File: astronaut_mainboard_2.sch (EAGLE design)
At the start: 32 parts, among them IC1 ADUM1250, IC2 741G3157DBVR, IC3 741G3157DBVR, J1 User Interface (I2C), J2 Arduino Mega (UART), J3 HF Comm (UART), J4 User Interface (I2C), J5 GNSS (UART), Q1 BSS138, Q2 BSS138, Q3 BSS138, Q4 BSS138

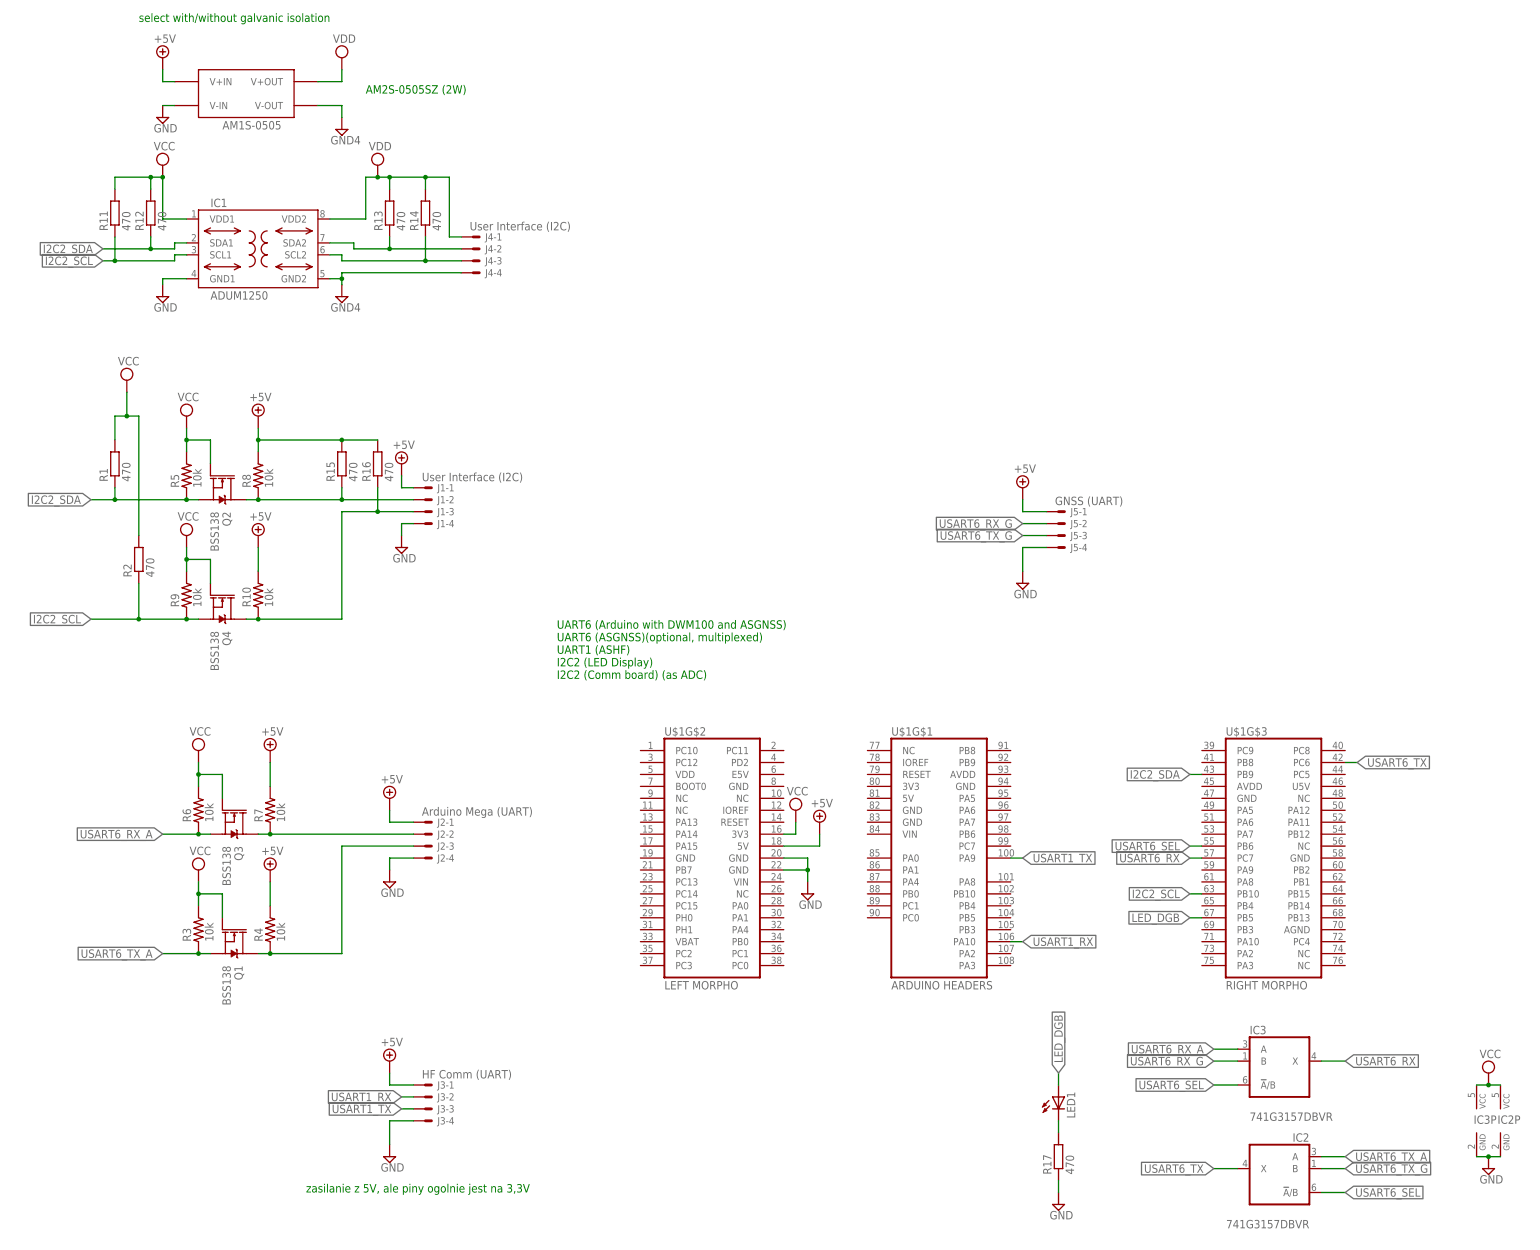
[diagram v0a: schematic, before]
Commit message: minor updates
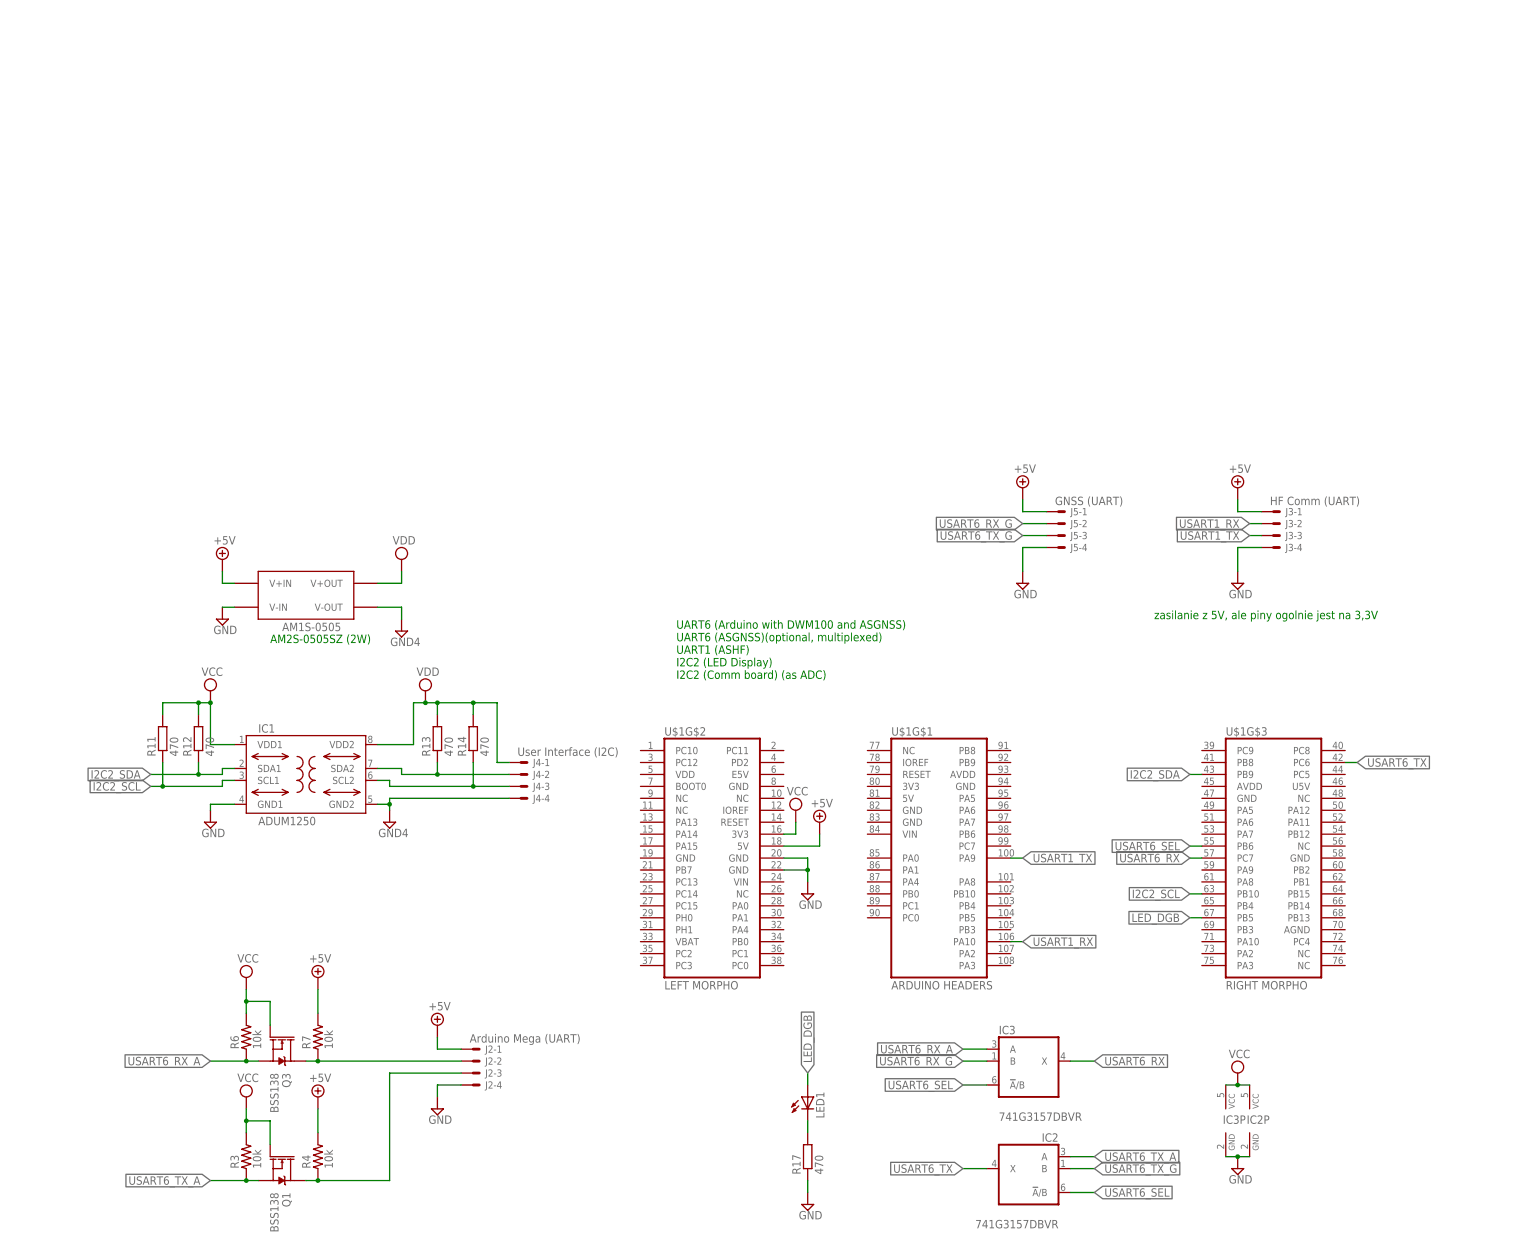
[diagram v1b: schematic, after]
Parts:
- removed J1: User Interface (I2C), EP_molex_6410_7395:22-05-7048-04
- removed Q2, Q4: BSS138, SparkFun-DiscreteSemi:MOSFET-NCH-AO3404A
- removed R1, R15, R16, R2: 470, rcl:R-EU_R0805
- removed R10, R5, R8, R9: 10k, rc-master-smd:R_1206
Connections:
- removed net ARDU_PIN_3: J1-2.S, Q2.D, R15.1, R8.1
- removed net ARDU_PIN_4: J1-3.S, Q4.D, R10.1, R16.1
- net +5V: no longer J1-1.S, R10.2, R15.2, R16.2, R8.2
- net GND: no longer J1-4.S
- net I2C2_SCL: no longer Q4.S, R2.1, R9.1
- net I2C2_SDA: no longer Q2.S, R1.1, R5.1
- net VCC: no longer Q2.G, Q4.G, R1.2, R2.2, R5.2, R9.2
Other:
- note removed: "select with/without galvanic isolation"
- moved on the sheet: IC1, IC2, IC2P, IC3, IC3P, J2-1, J2-2, J2-3, J2-4, J3-1, J3-2, J3-3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
